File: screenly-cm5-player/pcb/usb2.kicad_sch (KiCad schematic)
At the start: 8 parts, among them J7 10.0 QHHTZB6.3, U7 AP22652W6-7

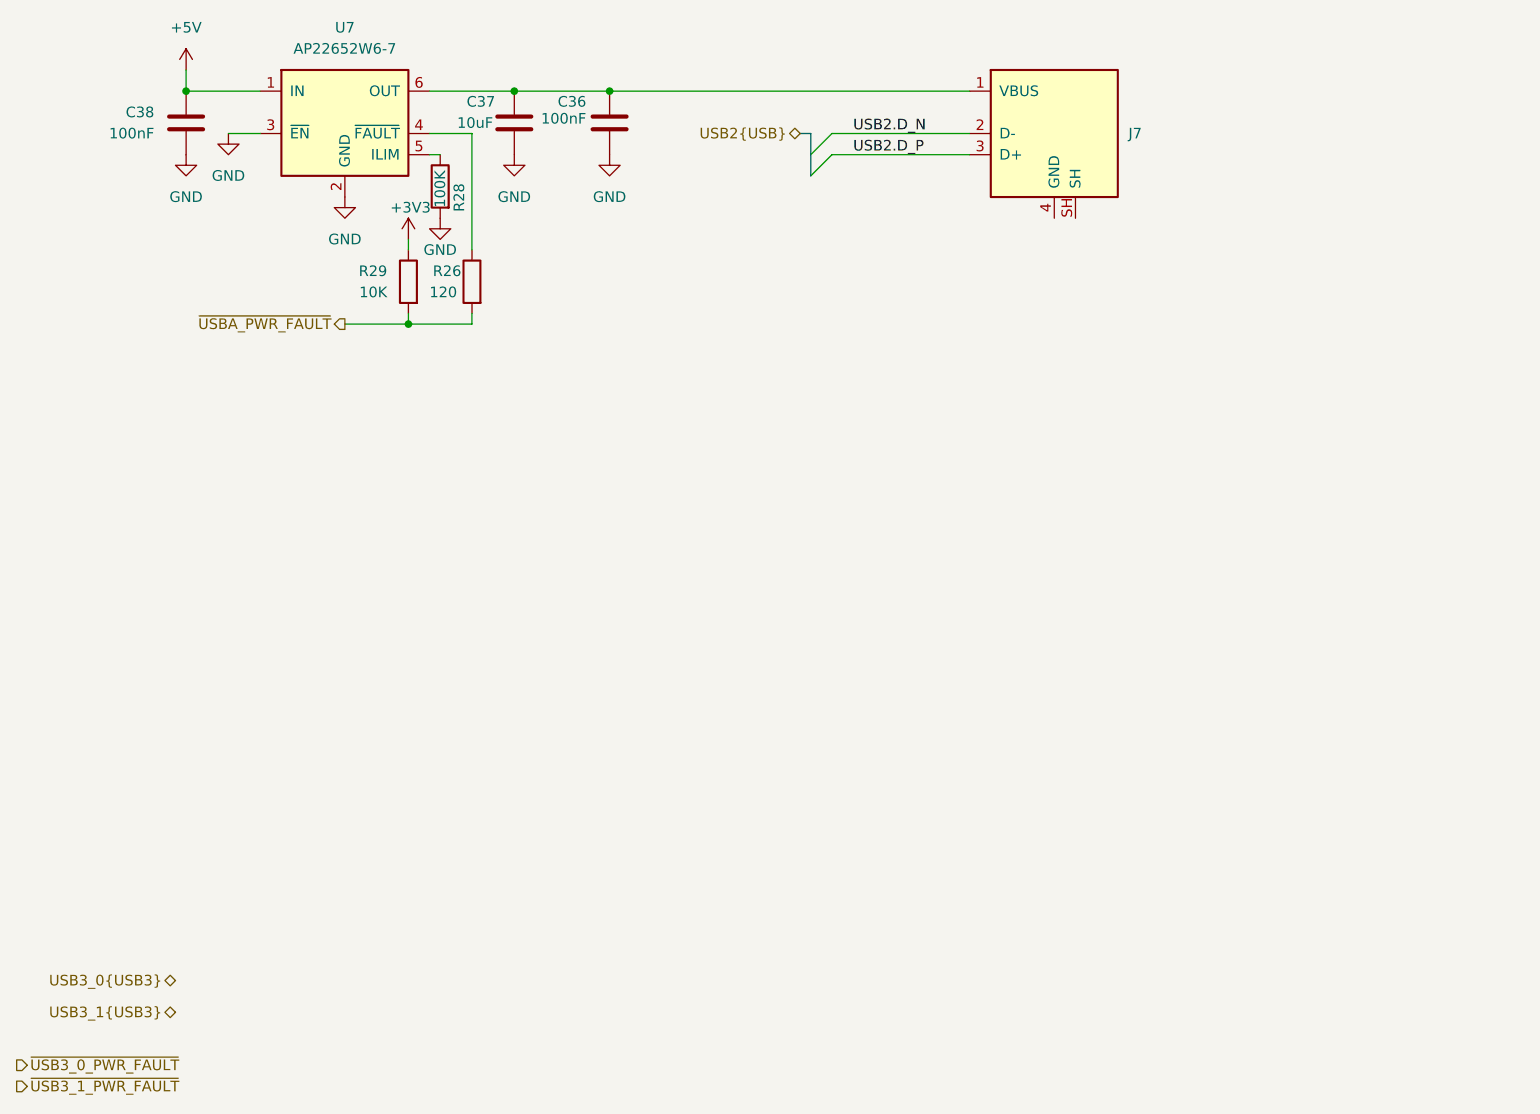
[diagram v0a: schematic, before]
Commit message: Finished USB
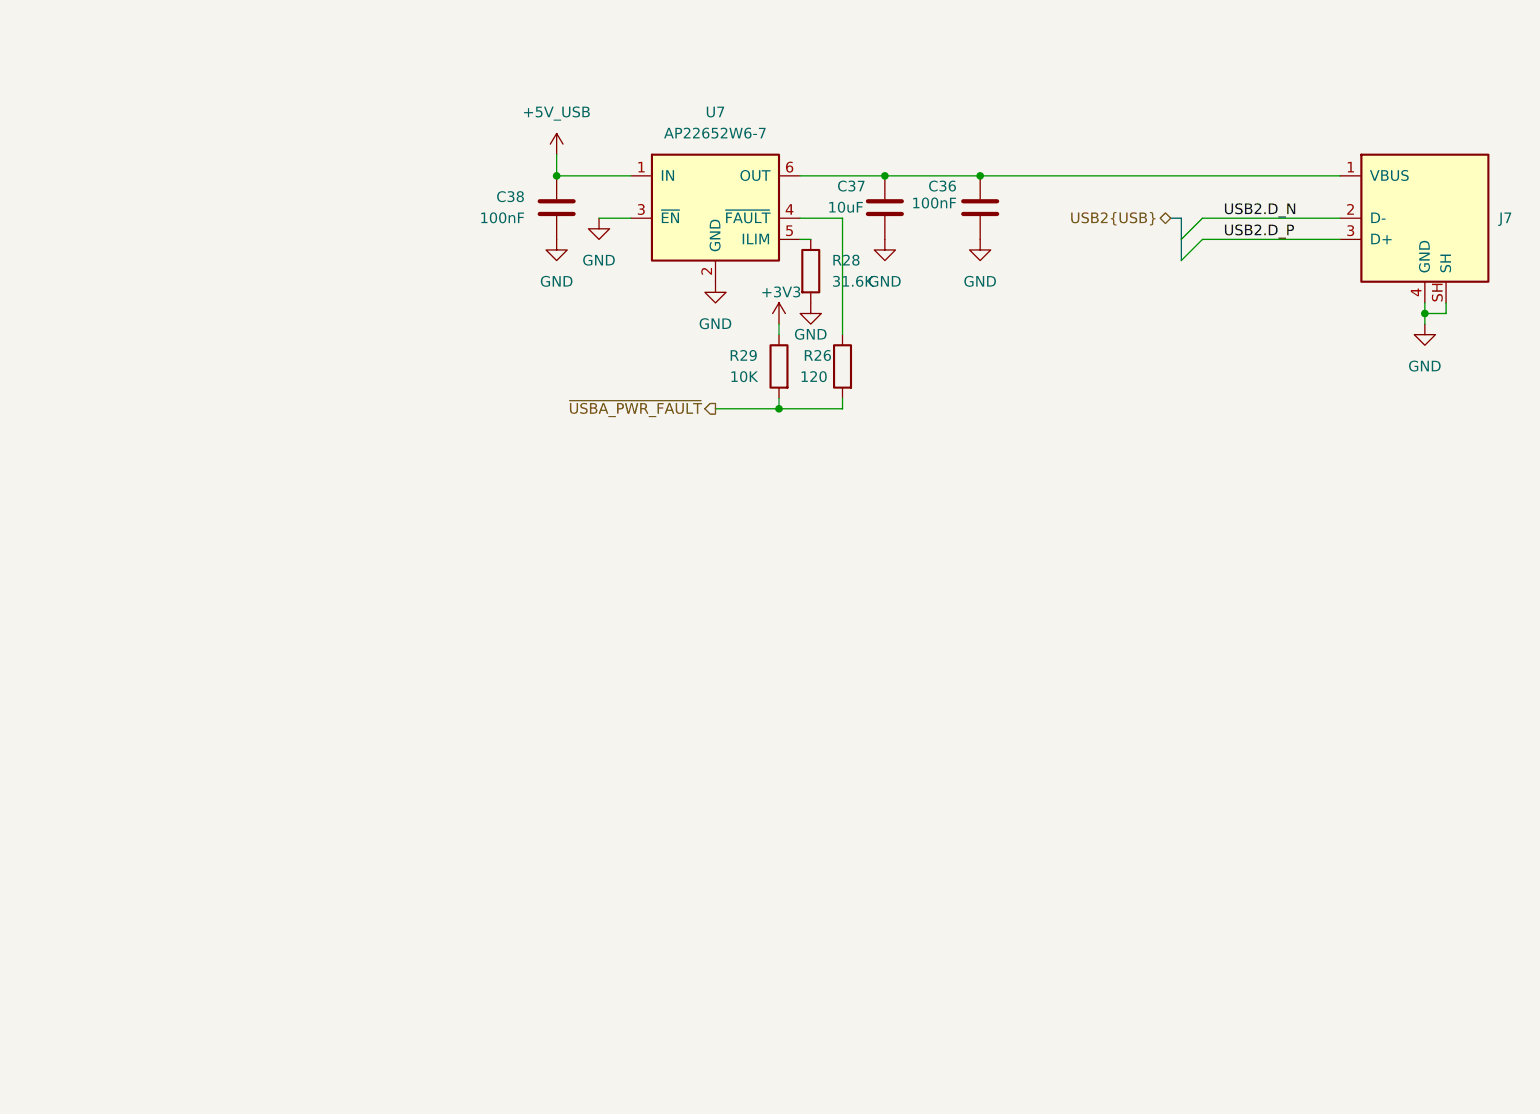
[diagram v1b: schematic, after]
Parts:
- removed R28: 100K, Screenly:R_0402, symbol Screenly:Resistor 100K 1% 0402 (0402WGF1003TCE)
- added R28: 31.6K, Screenly:R_0402, symbol Screenly:Resistor 31.6K 1% 0402 (0402WGF3162TCE)
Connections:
- net GND: now also J7.4 (GND), J7.SH, R28.2
- net at U7.5 (ILIM): now also R28.1
- net +5V renamed +5V_USB
